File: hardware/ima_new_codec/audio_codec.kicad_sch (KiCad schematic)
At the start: 19 parts, among them IC1 TLV320AIC3204IRHBR, J2 AudioJack2, J3 AudioJack2, J4 AudioJack2, J5 AudioJack2

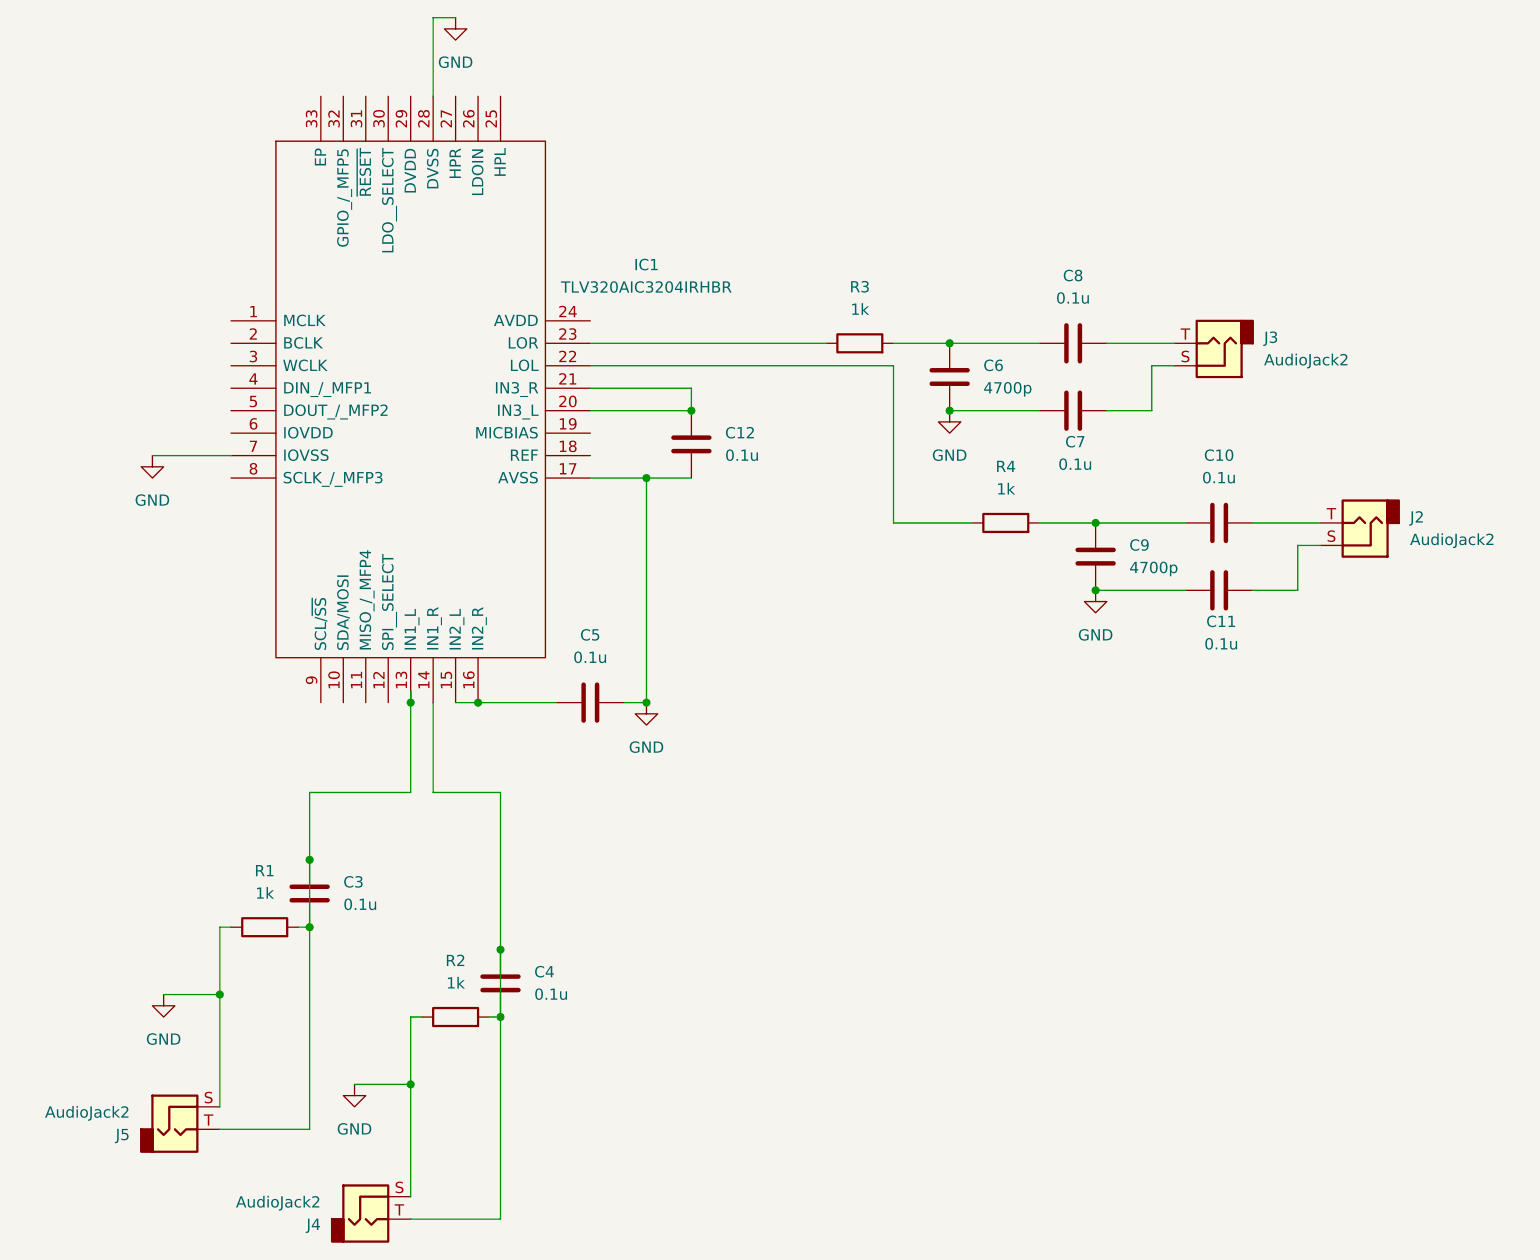
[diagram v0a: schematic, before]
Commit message: changes to input/output stages
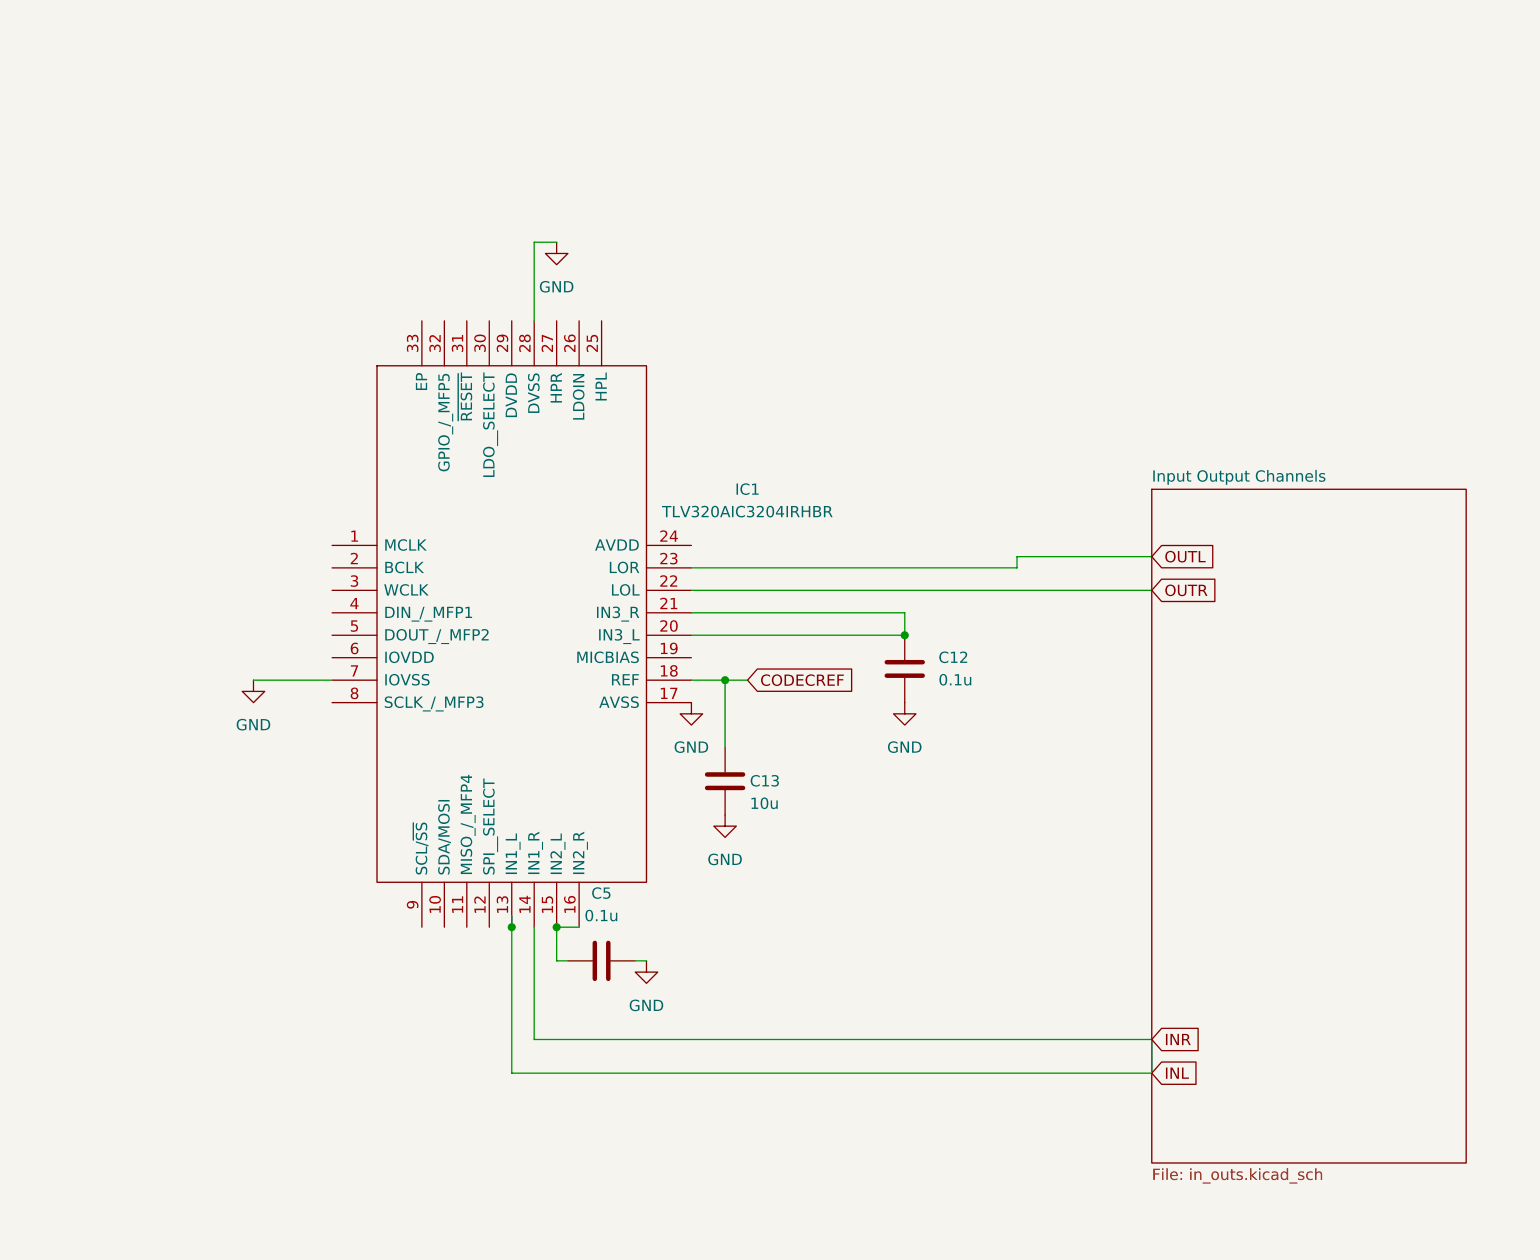
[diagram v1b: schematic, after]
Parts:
- removed C10, C11, C3, C4, C7, C8: 0.1u, symbol Device:C
- removed C6, C9: 4700p, symbol Device:C
- removed J2, J3, J4, J5: AudioJack2, symbol Connector_Audio:AudioJack2
- removed R1, R2, R3, R4: 1k, symbol Device:R
- added C13: 10u, symbol Device:C
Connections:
- net GND: now also C13.1
- net INL: now reaches IC1.14 (IN1_R)
- net INL: now also IC1.13 (IN1_L)
- net OUTL: now reaches IC1.23 (LOR)
- net OUTR: now reaches IC1.22 (LOL)
- net CODECREF: now reaches IC1.18 (REF)
- net CODECREF: now also C13.2
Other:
- added sheet Input Output Channels (in_outs.kicad_sch)
- moved on the sheet: C12, C5, IC1
